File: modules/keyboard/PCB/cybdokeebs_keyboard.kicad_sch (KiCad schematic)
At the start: 127 parts, among them SW1 SW_Push, SW10 SW_Push, SW11 SW_Push, SW12 SW_Push, SW13 SW_Push, SW14 SW_Push, SW15 SW_Push, SW16 SW_Push, SW17 SW_Push, SW18 SW_Push, SW19 SW_Push, SW2 SW_Push, SW20 SW_Push, SW21 SW_Push, SW22 SW_Push, SW23 SW_Push, SW24 SW_Push, SW25 SW_Push, SW26 SW_Push, SW27 SW_Push, SW28 SW_Push, SW29 SW_Push, SW3 SW_Push, SW30 SW_Push, SW31 SW_Push, SW32 SW_Push, SW33 SW_Push, SW34 SW_Push, SW35 SW_Push, SW36 SW_Push, SW37 SW_Push, SW38 SW_Push, SW39 SW_Push, SW4 SW_Push, SW40 SW_Push, SW41 SW_Push, SW42 SW_Push, SW43 SW_Push, SW44 SW_Push, SW45 SW_Push, SW46 SW_Push, SW47 SW_Push, SW48 SW_Push, SW49 SW_Push, SW5 SW_Push, SW50 SW_Push, SW51 SW_Push, SW52 SW_Push, SW53 SW_Push, SW54 SW_Push, SW55 SW_Push, SW56 SW_Push, SW57 SW_Push, SW58 SW_Push, SW59 SW_Push, SW6 SW_Push, SW60 SW_Push, SW61 SW_Push, SW7 SW_Push, SW8 SW_Push, SW9 SW_Push

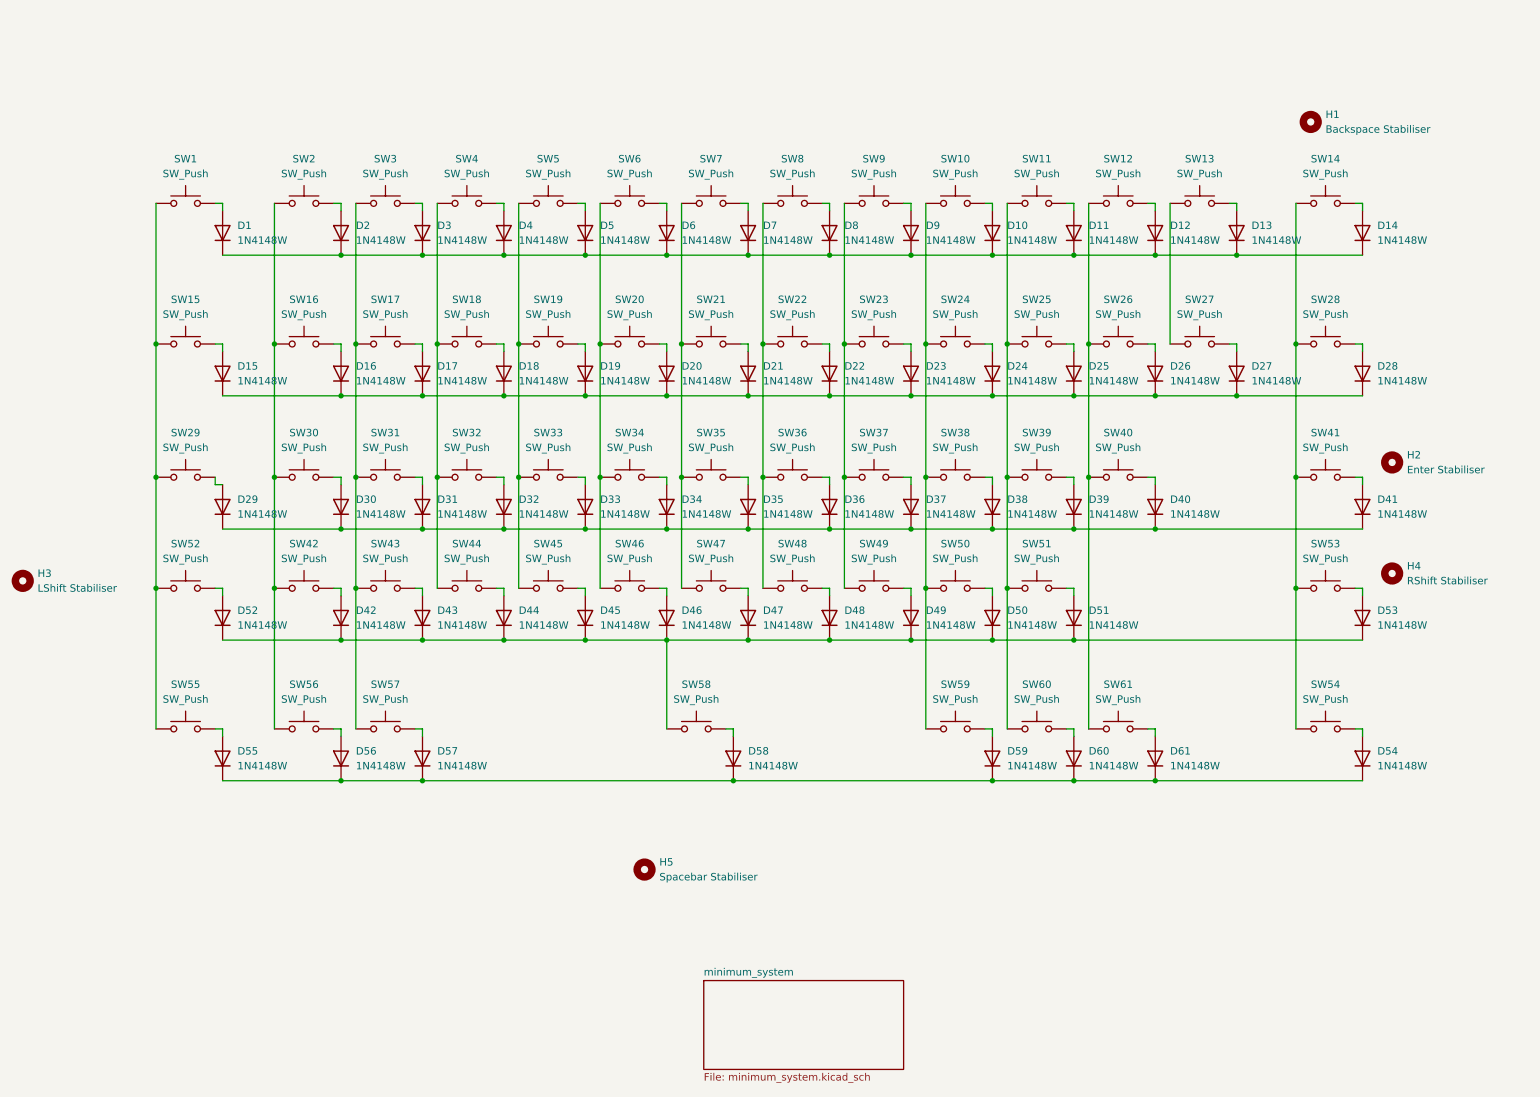
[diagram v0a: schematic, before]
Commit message: kb mostly done
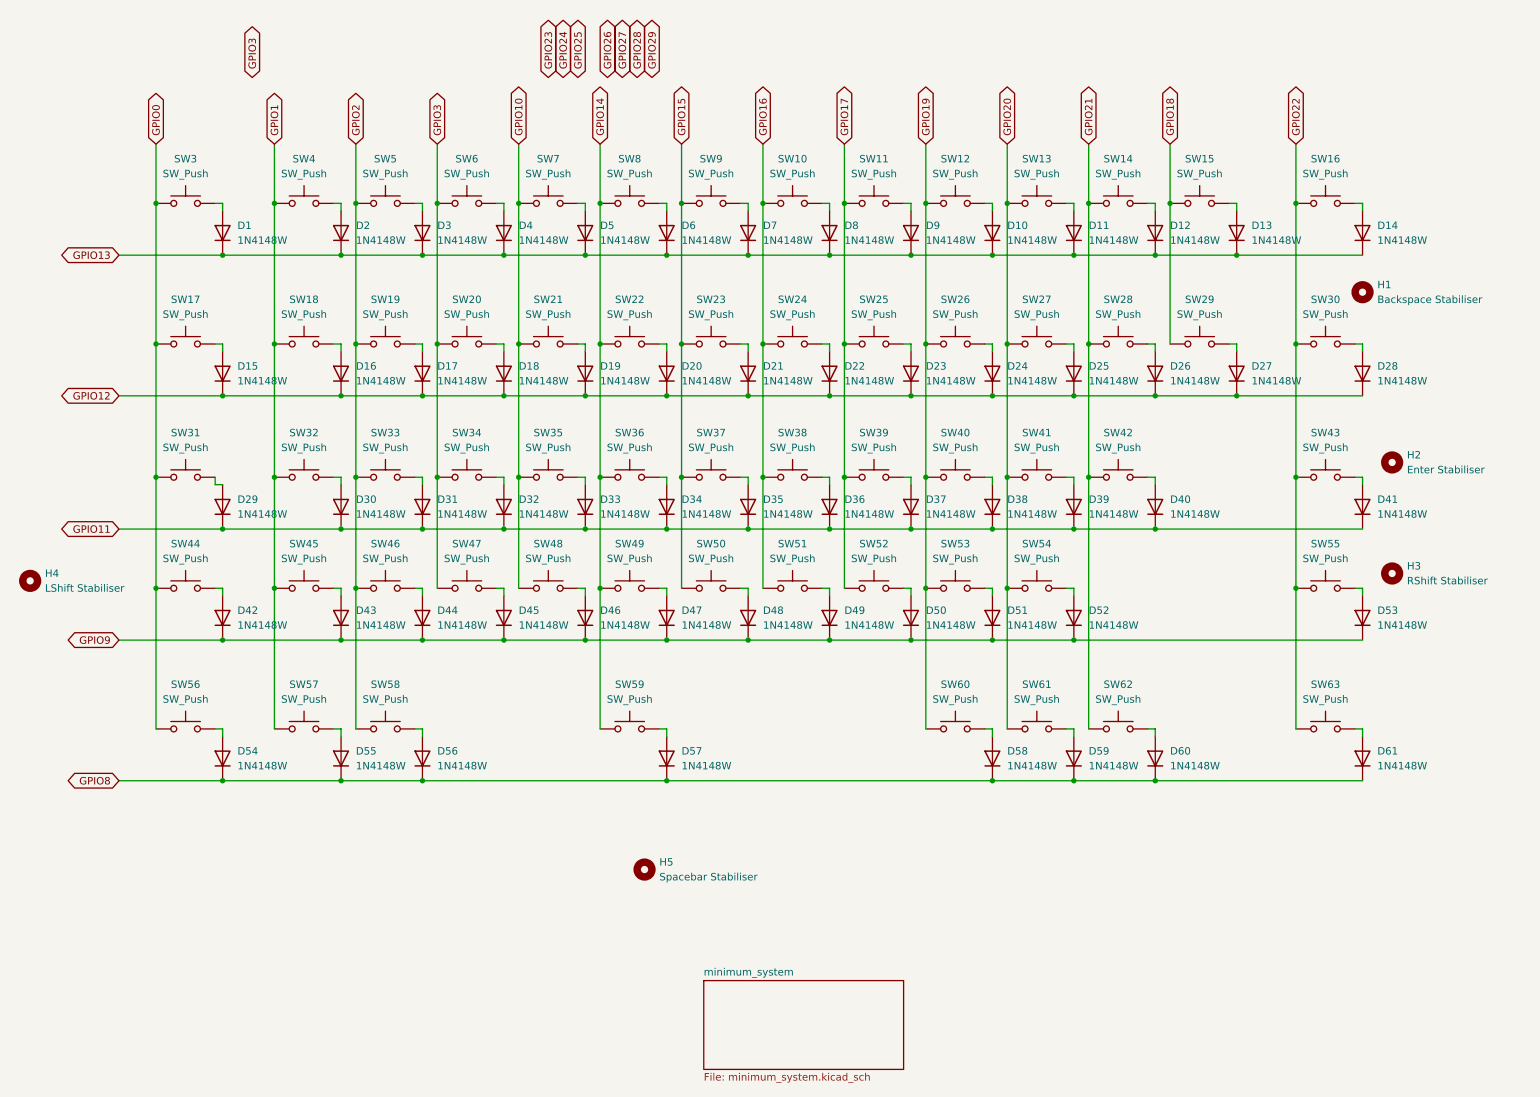
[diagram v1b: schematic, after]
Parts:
- SW10: renamed from SW8; footprint PCM_Switch_Keyboard_Hotswap_Kailh:SW_Hotswap_Kailh_MX_plated_1.00u -> PCM_Switch_Keyboard_Hotswap_Kailh:SW_Hotswap_Kailh_MX_1.00u
- SW11: renamed from SW9; footprint PCM_Switch_Keyboard_Hotswap_Kailh:SW_Hotswap_Kailh_MX_plated_1.00u -> PCM_Switch_Keyboard_Hotswap_Kailh:SW_Hotswap_Kailh_MX_1.00u
- SW12: renamed from SW10; footprint PCM_Switch_Keyboard_Hotswap_Kailh:SW_Hotswap_Kailh_MX_plated_1.00u -> PCM_Switch_Keyboard_Hotswap_Kailh:SW_Hotswap_Kailh_MX_1.00u
- SW13: renamed from SW11; footprint PCM_Switch_Keyboard_Hotswap_Kailh:SW_Hotswap_Kailh_MX_plated_1.00u -> PCM_Switch_Keyboard_Hotswap_Kailh:SW_Hotswap_Kailh_MX_1.00u
- SW14: renamed from SW12; footprint PCM_Switch_Keyboard_Hotswap_Kailh:SW_Hotswap_Kailh_MX_plated_1.00u -> PCM_Switch_Keyboard_Hotswap_Kailh:SW_Hotswap_Kailh_MX_1.00u
- SW15: renamed from SW13; footprint PCM_Switch_Keyboard_Hotswap_Kailh:SW_Hotswap_Kailh_MX_plated_1.00u -> PCM_Switch_Keyboard_Hotswap_Kailh:SW_Hotswap_Kailh_MX_1.00u
- SW16: renamed from SW14; footprint PCM_Switch_Keyboard_Hotswap_Kailh:SW_Hotswap_Kailh_MX_plated_1.00u -> PCM_Switch_Keyboard_Hotswap_Kailh:SW_Hotswap_Kailh_MX_2.00u
- SW17: renamed from SW15; footprint PCM_Switch_Keyboard_Hotswap_Kailh:SW_Hotswap_Kailh_MX_plated_1.00u -> PCM_Switch_Keyboard_Hotswap_Kailh:SW_Hotswap_Kailh_MX_1.50u
- SW18: renamed from SW16; footprint PCM_Switch_Keyboard_Hotswap_Kailh:SW_Hotswap_Kailh_MX_plated_2.00u -> PCM_Switch_Keyboard_Hotswap_Kailh:SW_Hotswap_Kailh_MX_1.00u
- SW19: renamed from SW17; footprint PCM_Switch_Keyboard_Hotswap_Kailh:SW_Hotswap_Kailh_MX_plated_1.50u -> PCM_Switch_Keyboard_Hotswap_Kailh:SW_Hotswap_Kailh_MX_1.00u
- SW20: renamed from SW18; footprint PCM_Switch_Keyboard_Hotswap_Kailh:SW_Hotswap_Kailh_MX_plated_1.00u -> PCM_Switch_Keyboard_Hotswap_Kailh:SW_Hotswap_Kailh_MX_1.00u
- SW21: renamed from SW19; footprint PCM_Switch_Keyboard_Hotswap_Kailh:SW_Hotswap_Kailh_MX_plated_1.00u -> PCM_Switch_Keyboard_Hotswap_Kailh:SW_Hotswap_Kailh_MX_1.00u
- SW22: renamed from SW20; footprint PCM_Switch_Keyboard_Hotswap_Kailh:SW_Hotswap_Kailh_MX_plated_1.00u -> PCM_Switch_Keyboard_Hotswap_Kailh:SW_Hotswap_Kailh_MX_1.00u
- SW23: renamed from SW21; footprint PCM_Switch_Keyboard_Hotswap_Kailh:SW_Hotswap_Kailh_MX_plated_1.00u -> PCM_Switch_Keyboard_Hotswap_Kailh:SW_Hotswap_Kailh_MX_1.00u
- SW24: renamed from SW22; footprint PCM_Switch_Keyboard_Hotswap_Kailh:SW_Hotswap_Kailh_MX_plated_1.00u -> PCM_Switch_Keyboard_Hotswap_Kailh:SW_Hotswap_Kailh_MX_1.00u
- SW25: renamed from SW23; footprint PCM_Switch_Keyboard_Hotswap_Kailh:SW_Hotswap_Kailh_MX_plated_1.00u -> PCM_Switch_Keyboard_Hotswap_Kailh:SW_Hotswap_Kailh_MX_1.00u
- SW26: renamed from SW24; footprint PCM_Switch_Keyboard_Hotswap_Kailh:SW_Hotswap_Kailh_MX_plated_1.00u -> PCM_Switch_Keyboard_Hotswap_Kailh:SW_Hotswap_Kailh_MX_1.00u
- SW27: renamed from SW25; footprint PCM_Switch_Keyboard_Hotswap_Kailh:SW_Hotswap_Kailh_MX_plated_1.00u -> PCM_Switch_Keyboard_Hotswap_Kailh:SW_Hotswap_Kailh_MX_1.00u
- SW28: renamed from SW26; footprint PCM_Switch_Keyboard_Hotswap_Kailh:SW_Hotswap_Kailh_MX_plated_1.00u -> PCM_Switch_Keyboard_Hotswap_Kailh:SW_Hotswap_Kailh_MX_1.00u
- SW29: renamed from SW27; footprint PCM_Switch_Keyboard_Hotswap_Kailh:SW_Hotswap_Kailh_MX_plated_1.00u -> PCM_Switch_Keyboard_Hotswap_Kailh:SW_Hotswap_Kailh_MX_1.00u
- SW3: renamed from SW1; footprint Button_Switch_SMD:SW_Push_SPST_NO_Alps_SKRK -> PCM_Switch_Keyboard_Hotswap_Kailh:SW_Hotswap_Kailh_MX_1.00u
- SW30: renamed from SW28; footprint PCM_Switch_Keyboard_Hotswap_Kailh:SW_Hotswap_Kailh_MX_plated_1.00u -> PCM_Switch_Keyboard_Hotswap_Kailh:SW_Hotswap_Kailh_MX_1.50u
- SW31: renamed from SW29; footprint PCM_Switch_Keyboard_Hotswap_Kailh:SW_Hotswap_Kailh_MX_plated_1.00u -> PCM_Switch_Keyboard_Hotswap_Kailh:SW_Hotswap_Kailh_MX_1.75u
- SW32: renamed from SW30; footprint PCM_Switch_Keyboard_Hotswap_Kailh:SW_Hotswap_Kailh_MX_plated_1.00u -> PCM_Switch_Keyboard_Hotswap_Kailh:SW_Hotswap_Kailh_MX_1.00u
- SW33: renamed from SW31; footprint PCM_Switch_Keyboard_Hotswap_Kailh:SW_Hotswap_Kailh_MX_plated_1.75u -> PCM_Switch_Keyboard_Hotswap_Kailh:SW_Hotswap_Kailh_MX_1.00u
- SW34: renamed from SW32; footprint PCM_Switch_Keyboard_Hotswap_Kailh:SW_Hotswap_Kailh_MX_plated_1.00u -> PCM_Switch_Keyboard_Hotswap_Kailh:SW_Hotswap_Kailh_MX_1.00u
- SW35: renamed from SW33; footprint PCM_Switch_Keyboard_Hotswap_Kailh:SW_Hotswap_Kailh_MX_plated_1.00u -> PCM_Switch_Keyboard_Hotswap_Kailh:SW_Hotswap_Kailh_MX_1.00u
- SW36: renamed from SW34; footprint PCM_Switch_Keyboard_Hotswap_Kailh:SW_Hotswap_Kailh_MX_plated_1.00u -> PCM_Switch_Keyboard_Hotswap_Kailh:SW_Hotswap_Kailh_MX_1.00u
- SW37: renamed from SW35; footprint PCM_Switch_Keyboard_Hotswap_Kailh:SW_Hotswap_Kailh_MX_plated_1.00u -> PCM_Switch_Keyboard_Hotswap_Kailh:SW_Hotswap_Kailh_MX_1.00u
- SW38: renamed from SW36; footprint PCM_Switch_Keyboard_Hotswap_Kailh:SW_Hotswap_Kailh_MX_plated_1.00u -> PCM_Switch_Keyboard_Hotswap_Kailh:SW_Hotswap_Kailh_MX_1.00u
- SW39: renamed from SW37; footprint PCM_Switch_Keyboard_Hotswap_Kailh:SW_Hotswap_Kailh_MX_plated_1.00u -> PCM_Switch_Keyboard_Hotswap_Kailh:SW_Hotswap_Kailh_MX_1.00u
- SW4: renamed from SW2; footprint Button_Switch_SMD:SW_Push_SPST_NO_Alps_SKRK -> PCM_Switch_Keyboard_Hotswap_Kailh:SW_Hotswap_Kailh_MX_1.00u
- SW40: renamed from SW38; footprint PCM_Switch_Keyboard_Hotswap_Kailh:SW_Hotswap_Kailh_MX_plated_1.00u -> PCM_Switch_Keyboard_Hotswap_Kailh:SW_Hotswap_Kailh_MX_1.00u
- SW41: renamed from SW39; footprint PCM_Switch_Keyboard_Hotswap_Kailh:SW_Hotswap_Kailh_MX_plated_1.00u -> PCM_Switch_Keyboard_Hotswap_Kailh:SW_Hotswap_Kailh_MX_1.00u
- SW42: renamed from SW40; footprint PCM_Switch_Keyboard_Hotswap_Kailh:SW_Hotswap_Kailh_MX_plated_1.00u -> PCM_Switch_Keyboard_Hotswap_Kailh:SW_Hotswap_Kailh_MX_1.00u
- SW43: renamed from SW41; footprint PCM_Switch_Keyboard_Hotswap_Kailh:SW_Hotswap_Kailh_MX_plated_1.00u -> PCM_Switch_Keyboard_Hotswap_Kailh:SW_Hotswap_Kailh_MX_2.25u
- SW44: renamed from SW52; footprint PCM_Switch_Keyboard_Hotswap_Kailh:SW_Hotswap_Kailh_MX_plated_1.00u -> PCM_Switch_Keyboard_Hotswap_Kailh:SW_Hotswap_Kailh_MX_2.25u
- SW45: renamed from SW42; footprint PCM_Switch_Keyboard_Hotswap_Kailh:SW_Hotswap_Kailh_MX_plated_1.00u -> PCM_Switch_Keyboard_Hotswap_Kailh:SW_Hotswap_Kailh_MX_1.00u
- SW46: renamed from SW43; footprint PCM_Switch_Keyboard_Hotswap_Kailh:SW_Hotswap_Kailh_MX_plated_2.25u -> PCM_Switch_Keyboard_Hotswap_Kailh:SW_Hotswap_Kailh_MX_1.00u
- SW47: renamed from SW44; footprint PCM_Switch_Keyboard_Hotswap_Kailh:SW_Hotswap_Kailh_MX_plated_2.25u -> PCM_Switch_Keyboard_Hotswap_Kailh:SW_Hotswap_Kailh_MX_1.00u
- SW48: renamed from SW45; footprint PCM_Switch_Keyboard_Hotswap_Kailh:SW_Hotswap_Kailh_MX_plated_1.00u -> PCM_Switch_Keyboard_Hotswap_Kailh:SW_Hotswap_Kailh_MX_1.00u
- SW49: renamed from SW46; footprint PCM_Switch_Keyboard_Hotswap_Kailh:SW_Hotswap_Kailh_MX_plated_1.00u -> PCM_Switch_Keyboard_Hotswap_Kailh:SW_Hotswap_Kailh_MX_1.00u
- SW5: renamed from SW3; footprint PCM_Switch_Keyboard_Hotswap_Kailh:SW_Hotswap_Kailh_MX_plated_1.00u -> PCM_Switch_Keyboard_Hotswap_Kailh:SW_Hotswap_Kailh_MX_1.00u
- SW50: renamed from SW47; footprint PCM_Switch_Keyboard_Hotswap_Kailh:SW_Hotswap_Kailh_MX_plated_1.00u -> PCM_Switch_Keyboard_Hotswap_Kailh:SW_Hotswap_Kailh_MX_1.00u
- SW51: renamed from SW48; footprint PCM_Switch_Keyboard_Hotswap_Kailh:SW_Hotswap_Kailh_MX_plated_1.00u -> PCM_Switch_Keyboard_Hotswap_Kailh:SW_Hotswap_Kailh_MX_1.00u
- SW52: renamed from SW49; footprint PCM_Switch_Keyboard_Hotswap_Kailh:SW_Hotswap_Kailh_MX_plated_1.00u -> PCM_Switch_Keyboard_Hotswap_Kailh:SW_Hotswap_Kailh_MX_1.00u
- SW53: renamed from SW50; footprint PCM_Switch_Keyboard_Hotswap_Kailh:SW_Hotswap_Kailh_MX_plated_1.00u -> PCM_Switch_Keyboard_Hotswap_Kailh:SW_Hotswap_Kailh_MX_1.00u
- SW54: renamed from SW51; footprint PCM_Switch_Keyboard_Hotswap_Kailh:SW_Hotswap_Kailh_MX_plated_1.00u -> PCM_Switch_Keyboard_Hotswap_Kailh:SW_Hotswap_Kailh_MX_1.00u
- SW55: renamed from SW53; footprint PCM_Switch_Keyboard_Hotswap_Kailh:SW_Hotswap_Kailh_MX_plated_1.00u -> PCM_Switch_Keyboard_Hotswap_Kailh:SW_Hotswap_Kailh_MX_2.75u
- SW56: renamed from SW55; footprint PCM_Switch_Keyboard_Hotswap_Kailh:SW_Hotswap_Kailh_MX_plated_2.75u -> PCM_Switch_Keyboard_Hotswap_Kailh:SW_Hotswap_Kailh_MX_1.25u
- SW57: renamed from SW56; footprint PCM_Switch_Keyboard_Hotswap_Kailh:SW_Hotswap_Kailh_MX_plated_1.25u -> PCM_Switch_Keyboard_Hotswap_Kailh:SW_Hotswap_Kailh_MX_1.25u
- SW58: renamed from SW57; footprint PCM_Switch_Keyboard_Hotswap_Kailh:SW_Hotswap_Kailh_MX_plated_1.25u -> PCM_Switch_Keyboard_Hotswap_Kailh:SW_Hotswap_Kailh_MX_1.25u
- SW59: renamed from SW58; footprint PCM_Switch_Keyboard_Hotswap_Kailh:SW_Hotswap_Kailh_MX_plated_1.25u -> PCM_Switch_Keyboard_Hotswap_Kailh:SW_Hotswap_Kailh_MX_6.25u
- SW6: renamed from SW4; footprint PCM_Switch_Keyboard_Hotswap_Kailh:SW_Hotswap_Kailh_MX_plated_1.00u -> PCM_Switch_Keyboard_Hotswap_Kailh:SW_Hotswap_Kailh_MX_1.00u
- SW60: renamed from SW59; footprint PCM_Switch_Keyboard_Hotswap_Kailh:SW_Hotswap_Kailh_MX_plated_6.25u -> PCM_Switch_Keyboard_Hotswap_Kailh:SW_Hotswap_Kailh_MX_1.25u
- SW61: renamed from SW60; footprint PCM_Switch_Keyboard_Hotswap_Kailh:SW_Hotswap_Kailh_MX_plated_1.25u -> PCM_Switch_Keyboard_Hotswap_Kailh:SW_Hotswap_Kailh_MX_1.25u
- SW62: renamed from SW61; footprint PCM_Switch_Keyboard_Hotswap_Kailh:SW_Hotswap_Kailh_MX_plated_1.25u -> PCM_Switch_Keyboard_Hotswap_Kailh:SW_Hotswap_Kailh_MX_1.25u
- SW63: renamed from SW54; footprint PCM_Switch_Keyboard_Hotswap_Kailh:SW_Hotswap_Kailh_MX_plated_1.00u -> PCM_Switch_Keyboard_Hotswap_Kailh:SW_Hotswap_Kailh_MX_1.25u
- SW7: renamed from SW5; footprint PCM_Switch_Keyboard_Hotswap_Kailh:SW_Hotswap_Kailh_MX_plated_1.00u -> PCM_Switch_Keyboard_Hotswap_Kailh:SW_Hotswap_Kailh_MX_1.00u
- SW8: renamed from SW6; footprint PCM_Switch_Keyboard_Hotswap_Kailh:SW_Hotswap_Kailh_MX_plated_1.00u -> PCM_Switch_Keyboard_Hotswap_Kailh:SW_Hotswap_Kailh_MX_1.00u
- SW9: renamed from SW7; footprint PCM_Switch_Keyboard_Hotswap_Kailh:SW_Hotswap_Kailh_MX_plated_1.00u -> PCM_Switch_Keyboard_Hotswap_Kailh:SW_Hotswap_Kailh_MX_1.00u
- renumbered D52 to D42, D42 to D43, D43 to D44, D44 to D45, D45 to D46, D46 to D47, D47 to D48, D48 to D49, D49 to D50, D50 to D51, D51 to D52, D55 to D54, D56 to D55, D57 to D56, D58 to D57, D59 to D58, D60 to D59, D61 to D60, D54 to D61, H4 to H3, H3 to H4
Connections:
- net GPIO11: now reaches D29.1 (K), D30.1 (K), D31.1 (K), D32.1 (K), D33.1 (K), D34.1 (K), D35.1 (K), D36.1 (K), D37.1 (K), D38.1 (K), D39.1 (K), D40.1 (K), D41.1 (K)
- net GPIO12: now reaches D15.1 (K), D16.1 (K), D17.1 (K), D18.1 (K), D19.1 (K), D20.1 (K), D21.1 (K), D22.1 (K), D23.1 (K), D24.1 (K), D25.1 (K), D26.1 (K), D27.1 (K), D28.1 (K)
- net GPIO16: now reaches SW10.1, SW24.1, SW38.1, SW51.1
- net GPIO13: now reaches D1.1 (K), D10.1 (K), D11.1 (K), D12.1 (K), D13.1 (K), D14.1 (K), D2.1 (K), D3.1 (K), D4.1 (K), D5.1 (K), D6.1 (K), D7.1 (K), D8.1 (K), D9.1 (K)
- net GPIO18: now reaches SW15.1, SW29.1
- net GPIO2: now reaches SW19.1, SW33.1, SW46.1, SW5.1, SW58.1
- net GPIO9: now reaches D42.1 (K), D43.1 (K), D44.1 (K), D45.1 (K), D46.1 (K), D47.1 (K), D48.1 (K), D49.1 (K), D50.1 (K), D51.1 (K), D52.1 (K), D53.1 (K)
- net GPIO9: no longer SW59.1
- net GPIO19: now reaches SW12.1, SW26.1, SW40.1, SW53.1, SW60.1
- net GPIO3: now reaches SW20.1, SW34.1, SW47.1, SW6.1
- net GPIO17: now reaches SW11.1, SW25.1, SW39.1, SW52.1
- net GPIO14: now reaches SW22.1, SW36.1, SW49.1, SW8.1
- net GPIO14: now also SW59.1
- net GPIO1: now reaches SW18.1, SW32.1, SW4.1, SW45.1, SW57.1
- net GPIO20: now reaches SW13.1, SW27.1, SW41.1, SW54.1, SW61.1
- net GPIO0: now reaches SW17.1, SW3.1, SW31.1, SW44.1, SW56.1
- net GPIO22: now reaches SW16.1, SW30.1, SW43.1, SW55.1, SW63.1
- net GPIO8: now reaches D54.1 (K), D55.1 (K), D56.1 (K), D57.1 (K), D58.1 (K), D59.1 (K), D60.1 (K), D61.1 (K)
- net GPIO10: now reaches SW21.1, SW35.1, SW48.1, SW7.1
- net GPIO15: now reaches SW23.1, SW37.1, SW50.1, SW9.1
- net GPIO21: now reaches SW14.1, SW28.1, SW42.1, SW62.1
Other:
- moved on the sheet: D57, H1, H4, SW59

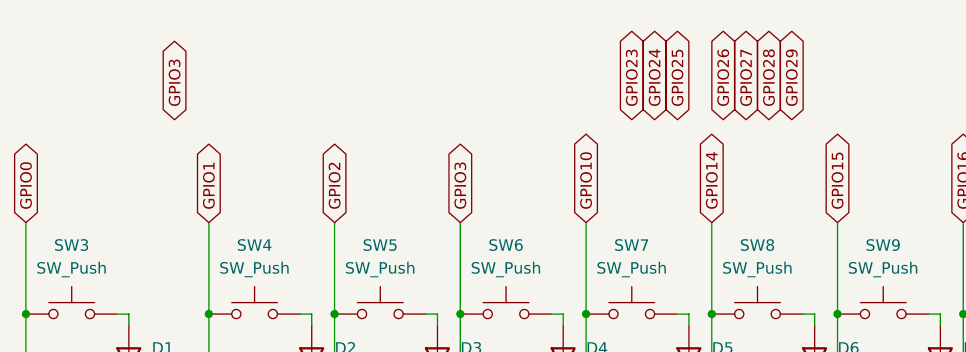
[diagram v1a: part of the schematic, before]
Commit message: finished all pcbs
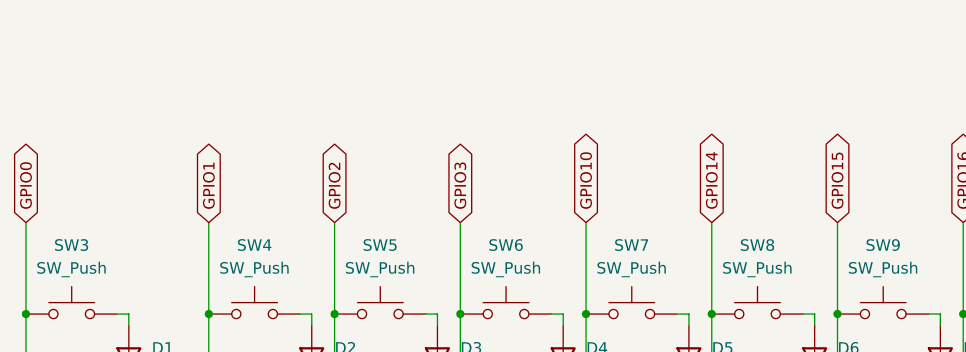
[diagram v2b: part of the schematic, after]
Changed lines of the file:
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@@
-		)
-	)
-	(global_label "GPIO28"
-		(shape bidirectional)
-		(at 128.27 22.86 90)
-		(fields_autoplaced yes)
-		(effects
-			(font
-				(size 1.27 1.27)
-			)
-			(justify left)
-		)
-		(property "Intersheetrefs" "${INTERSHEET_REFS}"
-			(at 128.27 11.8692 90)
-			(hide yes)
-			(show_name no)
-			(do_not_autoplace no)
-			(effects
-				(font
-					(size 1.27 1.27)
-				)
-				(justify left)
-			)
 		)
 	)
@@
 		)
 	)
-	(global_label "GPIO26"
-		(shape bidirectional)
-		(at 123.19 22.86 90)
-		(fields_autoplaced yes)
-		(effects
-			(font
-				(size 1.27 1.27)
-			)
-			(justify left)
-		)
-		(property "Intersheetrefs" "${INTERSHEET_REFS}"
-			(at 123.19 11.8692 90)
-			(hide yes)
-			(show_name no)
-			(do_not_autoplace no)
-			(effects
-				(font
-					(size 1.27 1.27)
-				)
-				(justify left)
-			)
-		)
-	)
 	(global_label "GPIO20"
 		(shape bidirectional)
@@
 		)
 	)
-	(global_label "GPIO3"
-		(shape bidirectional)
-		(at 62.23 22.86 90)
-		(fields_autoplaced yes)
-		(effects
-			(font
-				(size 1.27 1.27)
-			)
-			(justify left)
-		)
-		(property "Intersheetrefs" "${INTERSHEET_REFS}"
-			(at 62.23 13.0787 90)
-			(hide yes)
-			(show_name no)
-			(do_not_autoplace no)
-			(effects
-				(font
-					(size 1.27 1.27)
-				)
-				(justify left)
-			)
-		)
-	)
 	(global_label "GPIO9"
 		(shape bidirectional)
@@
 		)
 	)
-	(global_label "GPIO23"
-		(shape bidirectional)
-		(at 113.03 22.86 90)
-		(fields_autoplaced yes)
-		(effects
-			(font
-				(size 1.27 1.27)
-			)
-			(justify left)
-		)
-		(property "Intersheetrefs" "${INTERSHEET_REFS}"
-			(at 113.03 11.8692 90)
-			(hide yes)
-			(show_name no)
-			(do_not_autoplace no)
-			(effects
-				(font
-					(size 1.27 1.27)
-				)
-				(justify left)
-			)
-		)
-	)
 	(global_label "GPIO22"
 		(shape bidirectional)
@@
 		)
 	)
-	(global_label "GPIO24"
-		(shape bidirectional)
-		(at 115.57 22.86 90)
-		(fields_autoplaced yes)
-		(effects
-			(font
-				(size 1.27 1.27)
-			)
-			(justify left)
-		)
-		(property "Intersheetrefs" "${INTERSHEET_REFS}"
-			(at 115.57 11.8692 90)
-			(hide yes)
-			(show_name no)
-			(do_not_autoplace no)
-			(effects
-				(font
-					(size 1.27 1.27)
-				)
-				(justify left)
-			)
-		)
-	)
-	(global_label "GPIO25"
-		(shape bidirectional)
-		(at 118.11 22.86 90)
-		(fields_autoplaced yes)
-		(effects
-			(font
-				(size 1.27 1.27)
-			)
-			(justify left)
-		)
-		(property "Intersheetrefs" "${INTERSHEET_REFS}"
-			(at 118.11 11.8692 90)
-			(hide yes)
-			(show_name no)
-			(do_not_autoplace no)
-			(effects
-				(font
-					(size 1.27 1.27)
-				)
-				(justify left)
-			)
-		)
-	)
 	(global_label "GPIO18"
 		(shape bidirectional)
@@
 			(hide yes)
 			(show_name no)
-			(do_not_autoplace no)
-			(effects
-				(font
-					(size 1.27 1.27)
-				)
-				(justify left)
-			)
-		)
-	)
-	(global_label "GPIO27"
-		(shape bidirectional)
-		(at 125.73 22.86 90)
-		(fields_autoplaced yes)
-		(effects
-			(font
-				(size 1.27 1.27)
-			)
-			(justify left)
-		)
-		(property "Intersheetrefs" "${INTERSHEET_REFS}"
-			(at 125.73 11.8692 90)
-			(hide yes)
-			(show_name no)
-			(do_not_autoplace no)
-			(effects
-				(font
-					(size 1.27 1.27)
-				)
-				(justify left)
-			)
-		)
-	)
-	(global_label "GPIO29"
-		(shape bidirectional)
-		(at 130.81 22.86 90)
-		(fields_autoplaced yes)
-		(effects
-			(font
-				(size 1.27 1.27)
-			)
-			(justify left)
-		)
-		(property "Intersheetrefs" "${INTERSHEET_REFS}"
-			(at 130.81 11.8692 90)
-			(hide yes)
-			(show_name no)
